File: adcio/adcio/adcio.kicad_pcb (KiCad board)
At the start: 2 copper layers, 48.3 x 50.8 mm, 4 parts, among them J3 RJ45_Shielded, J4 RJ45_Shielded

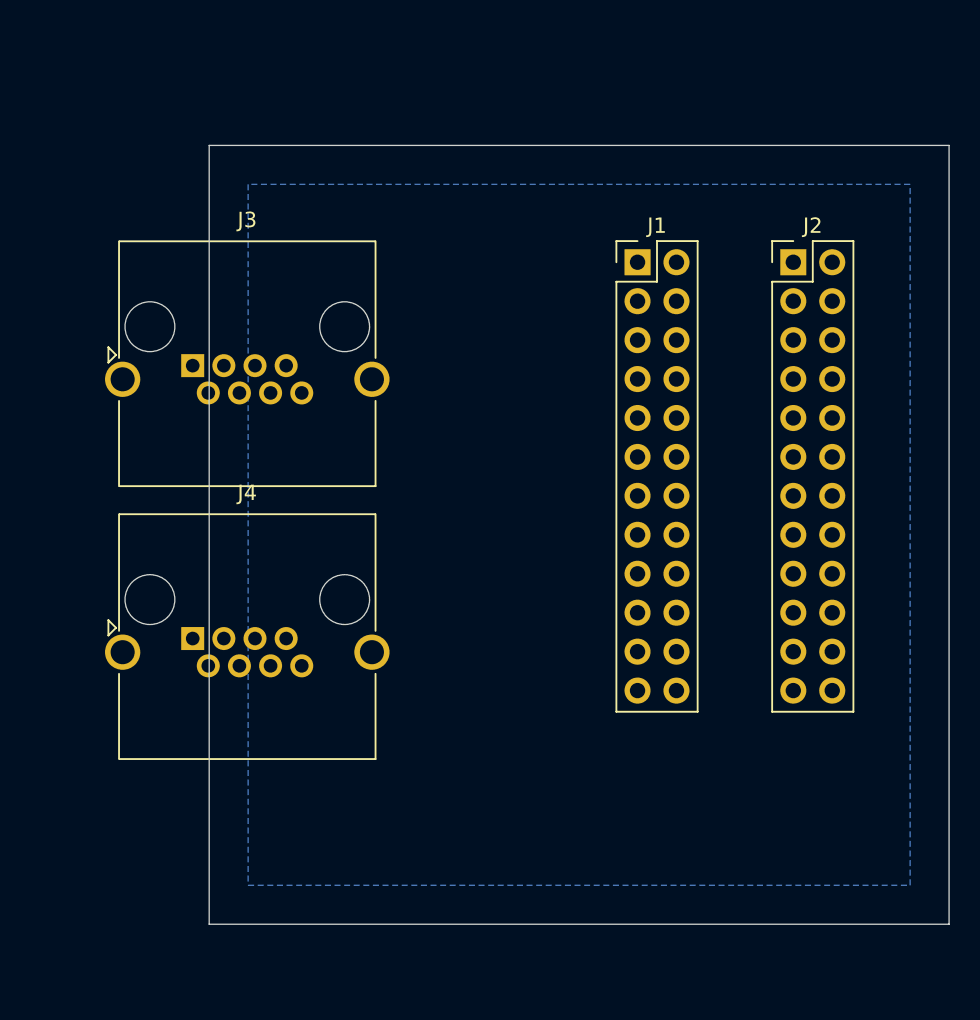
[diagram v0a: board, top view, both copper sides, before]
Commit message: ADCIO PCB done.
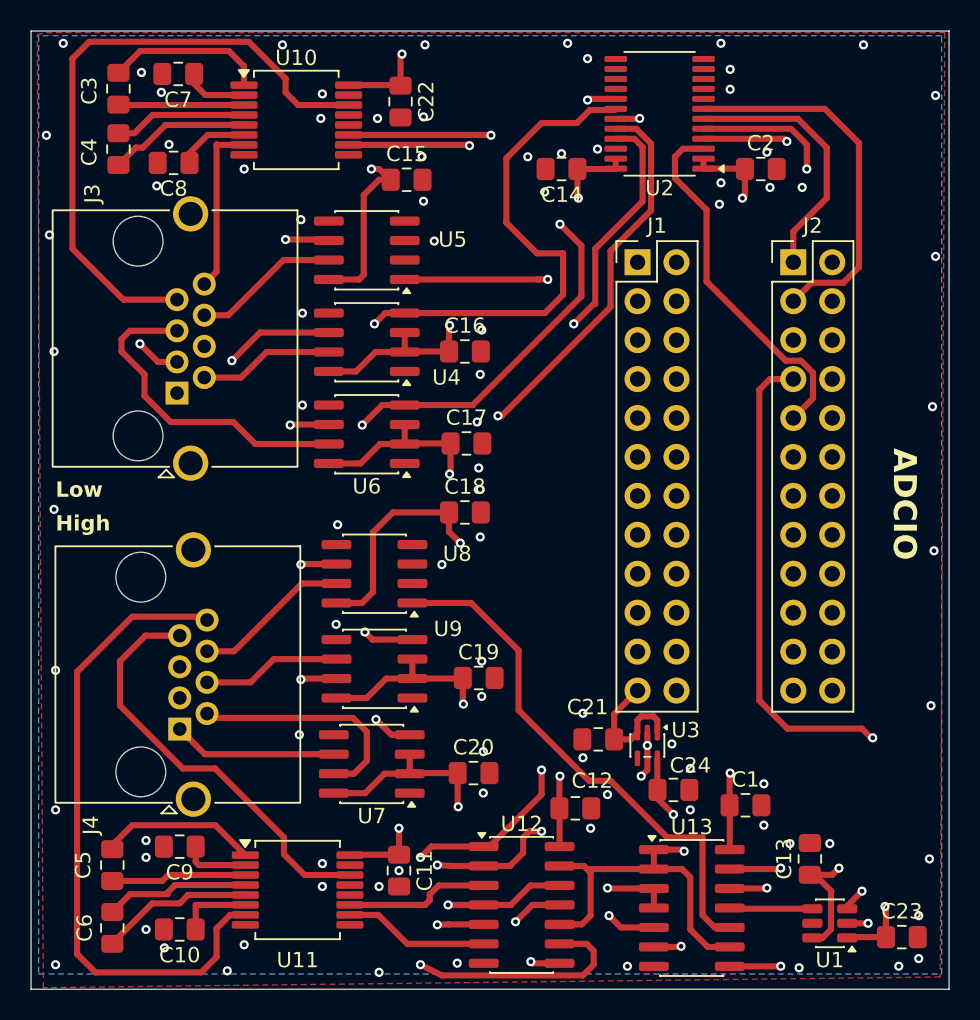
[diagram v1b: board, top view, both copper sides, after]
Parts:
- added C1: 100n, Capacitor_SMD:C_0805_2012Metric_Pad1.18x1.45mm_HandSolder, F.Cu at (182.3, 116.7)
- added C10: 100n, Capacitor_SMD:C_0805_2012Metric_Pad1.18x1.45mm_HandSolder, F.Cu at (145.4, 124.8)
- added C11: 100n, Capacitor_SMD:C_0805_2012Metric_Pad1.18x1.45mm_HandSolder, F.Cu at (159.7, 121.0)
- added C12: 100n, Capacitor_SMD:C_0805_2012Metric_Pad1.18x1.45mm_HandSolder, F.Cu at (171.2, 116.9)
- added C13: 100n, Capacitor_SMD:C_0805_2012Metric_Pad1.18x1.45mm_HandSolder, F.Cu at (186.5, 120.2)
- added C14: 100n, Capacitor_SMD:C_0805_2012Metric_Pad1.18x1.45mm_HandSolder, F.Cu at (170.3, 75.2)
- added C15: 100n, Capacitor_SMD:C_0805_2012Metric_Pad1.18x1.45mm_HandSolder, F.Cu at (160.2, 75.9)
- added C16: 100n, Capacitor_SMD:C_0805_2012Metric_Pad1.18x1.45mm_HandSolder, F.Cu at (164.0, 87.1)
- added C17: 100n, Capacitor_SMD:C_0805_2012Metric_Pad1.18x1.45mm_HandSolder, F.Cu at (164.1, 93.1)
- added C18: 100n, Capacitor_SMD:C_0805_2012Metric_Pad1.18x1.45mm_HandSolder, F.Cu at (164.0, 97.6)
- added C19: 100n, Capacitor_SMD:C_0805_2012Metric_Pad1.18x1.45mm_HandSolder, F.Cu at (164.9, 108.4)
- added C2: 100n, Capacitor_SMD:C_0805_2012Metric_Pad1.18x1.45mm_HandSolder, F.Cu at (183.3, 75.2)
- added C20: 100n, Capacitor_SMD:C_0805_2012Metric_Pad1.18x1.45mm_HandSolder, F.Cu at (164.6, 114.6)
- added C21: 100n, Capacitor_SMD:C_0805_2012Metric_Pad1.18x1.45mm_HandSolder, F.Cu at (172.7, 112.4)
- added C22: 100n, Capacitor_SMD:C_0805_2012Metric_Pad1.18x1.45mm_HandSolder, F.Cu at (159.8, 70.8)
- added C23: 100n, Capacitor_SMD:C_0805_2012Metric_Pad1.18x1.45mm_HandSolder, F.Cu at (192.5, 125.3)
- added C24: 100n, Capacitor_SMD:C_0805_2012Metric_Pad1.18x1.45mm_HandSolder, F.Cu at (177.6, 115.7)
- added C3: 100n, Capacitor_SMD:C_0805_2012Metric_Pad1.18x1.45mm_HandSolder, F.Cu at (141.4, 70.0)
- added C4: 100n, Capacitor_SMD:C_0805_2012Metric_Pad1.18x1.45mm_HandSolder, F.Cu at (141.4, 73.9)
- added C5: 100n, Capacitor_SMD:C_0805_2012Metric_Pad1.18x1.45mm_HandSolder, F.Cu at (141.0, 120.6)
- added C6: 100n, Capacitor_SMD:C_0805_2012Metric_Pad1.18x1.45mm_HandSolder, F.Cu at (141.0, 124.7)
- added C7: 100n, Capacitor_SMD:C_0805_2012Metric_Pad1.18x1.45mm_HandSolder, F.Cu at (145.3, 69.0)
- added C8: 100n, Capacitor_SMD:C_0805_2012Metric_Pad1.18x1.45mm_HandSolder, F.Cu at (145.0, 74.8)
- added C9: 100n, Capacitor_SMD:C_0805_2012Metric_Pad1.18x1.45mm_HandSolder, F.Cu at (145.4, 119.4)
- added U1: SN74LVC1T45DBV, Package_TO_SOT_SMD:SOT-23-6, F.Cu at (187.8, 124.4)
- added U10: MAX3232, Package_SO:SSOP-16_5.3x6.2mm_P0.65mm, F.Cu at (153.0, 72.0)
- added U11: MAX3232, Package_SO:SSOP-16_5.3x6.2mm_P0.65mm, F.Cu at (153.1, 122.2)
- added U12: 74LS32, Package_SO:SOIC-14_3.9x8.7mm_P1.27mm, F.Cu at (167.7, 123.2)
- added U13: 74LS00, Package_SO:SOIC-14_3.9x8.7mm_P1.27mm, F.Cu at (178.8, 123.4)
- added U2: SN74LVC8T245, Package_SO:TSSOP-24_4.4x7.8mm_P0.65mm, F.Cu at (176.7, 71.6)
- added U3: TLV70018_SOT353, Package_TO_SOT_SMD:SOT-353_SC-70-5, F.Cu at (175.9, 112.8)
- added U4: MAX3485, Package_SO:SOIC-8_3.9x4.9mm_P1.27mm, F.Cu at (157.6, 86.5)
- added U5: MAX3485, Package_SO:SOIC-8_3.9x4.9mm_P1.27mm, F.Cu at (157.6, 80.5)
- added U6: MAX3485, Package_SO:SOIC-8_3.9x4.9mm_P1.27mm, F.Cu at (157.6, 92.5)
- added U7: MAX3485, Package_SO:SOIC-8_3.9x4.9mm_P1.27mm, F.Cu at (157.9, 114.0)
- added U8: MAX3485, Package_SO:SOIC-8_3.9x4.9mm_P1.27mm, F.Cu at (158.1, 101.6)
- added U9: MAX3485, Package_SO:SOIC-8_3.9x4.9mm_P1.27mm, F.Cu at (158.1, 107.8)
- moved J4 5.97 mm to (145.4, 111.7), turned to 90 degrees
- moved J3 2.06 mm to (145.2, 89.8), turned to 90 degrees
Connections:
- J2 pad 1: unconnected-(J2-CLK-Pad1) -> Net-(J2-CLK)
- J2 pad 13: unconnected-(J2-CS1-Pad13) -> Net-(J2-CS1)
- J2 pad 15: unconnected-(J2-CS2-Pad15) -> Net-(J2-CS2)
- J2 pad 3: unconnected-(J2-DIN-Pad3) -> Net-(J2-DIN)
- J2 pad 7: unconnected-(J2-DOUT-Pad7) -> Net-(J2-DOUT)
- J2 pad 9: unconnected-(J2-CS0-Pad9) -> Net-(J2-CS0)
- J3 pad 1: unconnected-(J3-Pad1) -> Net-(U4-A)
- J3 pad 2: unconnected-(J3-Pad2) -> Net-(U4-B)
- J3 pad 3: unconnected-(J3-Pad3) -> Net-(U5-A)
- J3 pad 4: unconnected-(J3-Pad4) -> Net-(U6-A)
- J3 pad 5: unconnected-(J3-Pad5) -> Net-(U6-B)
- J3 pad 6: unconnected-(J3-Pad6) -> Net-(U5-B)
- J3 pad 7: unconnected-(J3-Pad7) -> Net-(U10-T1OUT)
- J3 pad 8: unconnected-(J3-Pad8) -> Net-(U10-T2OUT)
- J3 pad SH: unconnected-(J3-PadSH) -> GND
- J4 pad 1: unconnected-(J4-Pad1) -> Net-(U7-A)
- J4 pad 2: unconnected-(J4-Pad2) -> Net-(U7-B)
- J4 pad 3: unconnected-(J4-Pad3) -> Net-(U8-A)
- J4 pad 4: unconnected-(J4-Pad4) -> Net-(U9-A)
- J4 pad 5: unconnected-(J4-Pad5) -> Net-(U9-B)
- J4 pad 6: unconnected-(J4-Pad6) -> Net-(U8-B)
- J4 pad 7: unconnected-(J4-Pad7) -> Net-(U11-T1OUT)
- J4 pad 8: unconnected-(J4-Pad8) -> Net-(U11-T2OUT)
- J4 pad SH: unconnected-(J4-PadSH) -> GND
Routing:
- net 3.3v: track 0.00 -> 114.5 mm, vias 0 -> 12
- net SEL0: track 0.00 -> 78.4 mm, vias 0 -> 4
- net SEL2: track 0.00 -> 75.7 mm, vias 0 -> 2
- net Net-(U10-T1IN): track 0.00 -> 66.4 mm, vias 0 -> 2
- net SEL1: track 0.00 -> 65.8 mm, vias 0 -> 2
- net Net-(U10-T2IN): track 0.00 -> 63.1 mm, vias 0 -> 2
- net SPI_CLK: track 0.00 -> 61.4 mm, vias 0 -> 2
- net Net-(U5-RO): track 0.00 -> 57.0 mm, vias 0 -> 2
- net SPI_OUT: track 0.00 -> 50.6 mm, vias 0 -> 4
- net Net-(J2-DOUT): track 0.00 -> 43.0 mm, vias 0 -> 2
- net Net-(U11-T2OUT): track 0.00 -> 42.6 mm
- net Net-(U10-T1OUT): track 0.00 -> 41.3 mm
- net Net-(J2-CS2): track 0.00 -> 37.4 mm, vias 0 -> 1
- net Net-(U8-RO): track 0.00 -> 34.7 mm
- net Net-(U8-A): track 0.00 -> 31.5 mm, vias 0 -> 1
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- added copper zone on In1.Cu, net 1.8v
- added copper zone on In2.Cu, net 3.3v
- added copper zone on F.Cu, net GND
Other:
- board size 48.3 x 50.8 mm -> 59.9 x 62.5 mm
- copper layers 2 -> 4
- board text added: "ADCIO"
- board text added: "High"
- board text added: "Low"
